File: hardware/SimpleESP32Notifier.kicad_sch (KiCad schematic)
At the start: 1 part, among them U1 Heltec_HTIT-WB32

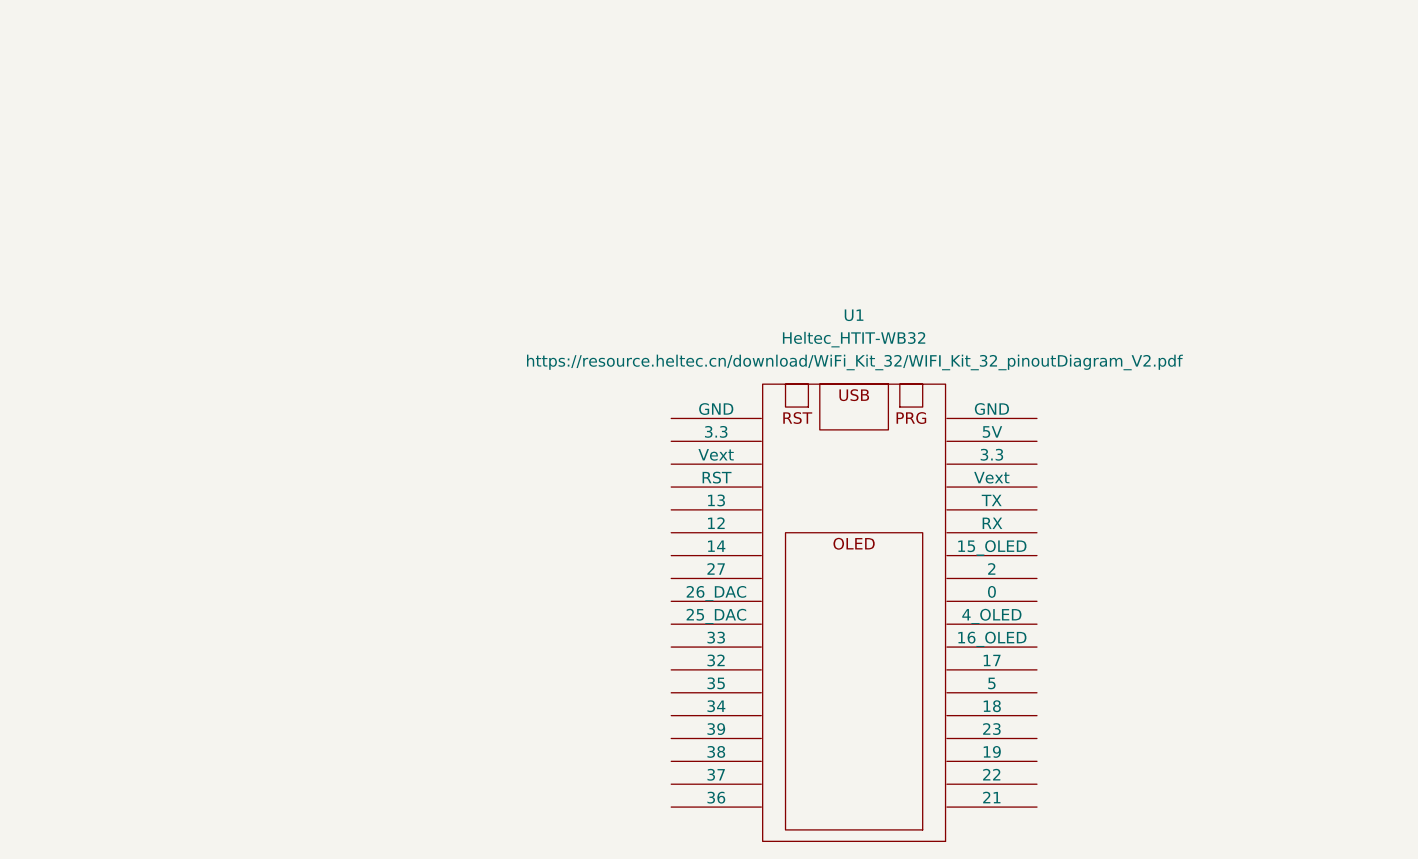
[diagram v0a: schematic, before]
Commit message: Decided layout
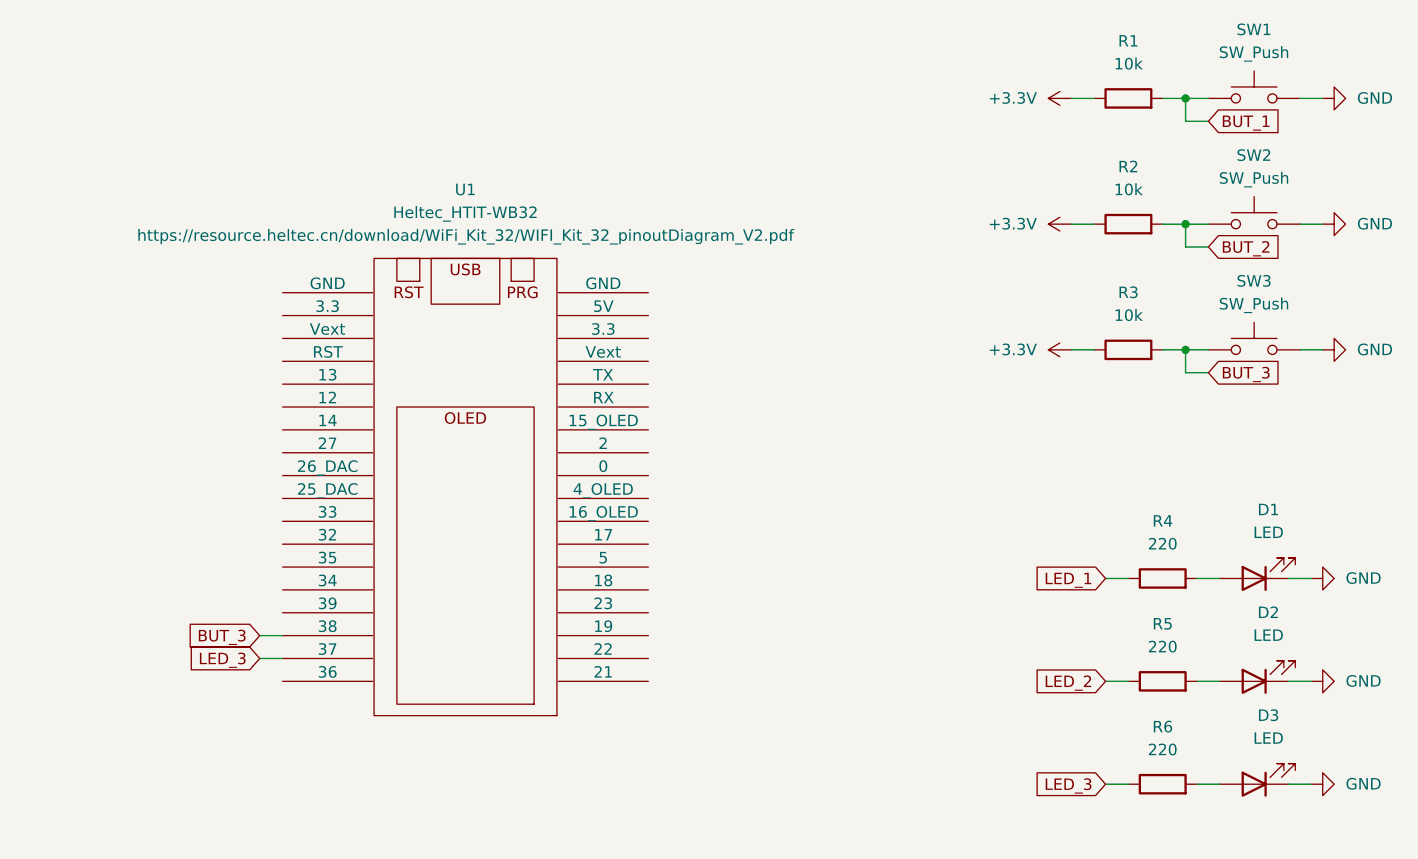
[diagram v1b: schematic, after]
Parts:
- added D1, D2, D3: LED, LED_THT:LED_D5.0mm, symbol Device:LED
- added R1, R2, R3: 10k, Resistor_THT:R_Axial_DIN0207_L6.3mm_D2.5mm_P7.62mm_Horizontal, symbol Device:R
- added R4, R5, R6: 220, Resistor_THT:R_Axial_DIN0207_L6.3mm_D2.5mm_P7.62mm_Horizontal, symbol Device:R
- added SW1, SW2, SW3: SW_Push, Button_Switch_THT:SW_PUSH_6mm, symbol Switch:SW_Push
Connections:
- net LED_3: now reaches U1.37
- net LED_3: now also R6.1
- net BUT_3: now reaches U1.38
- net BUT_3: now also R3.2, SW3.1
- new net: D1.2 (A), R4.2
- new net: D2.2 (A), R5.2
- new net: D3.2 (A), R6.2
- new net +3.3V: R1.1, R2.1, R3.1
- new net BUT_1: R1.2, SW1.1
- new net BUT_2: R2.2, SW2.1
- new net GND: D1.1 (K), D2.1 (K), D3.1 (K), SW1.2, SW2.2, SW3.2
- new net LED_1: R4.1
- new net LED_2: R5.1
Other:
- moved on the sheet: U1
